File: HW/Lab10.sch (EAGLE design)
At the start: 8 parts, among them Q1 IRLD024

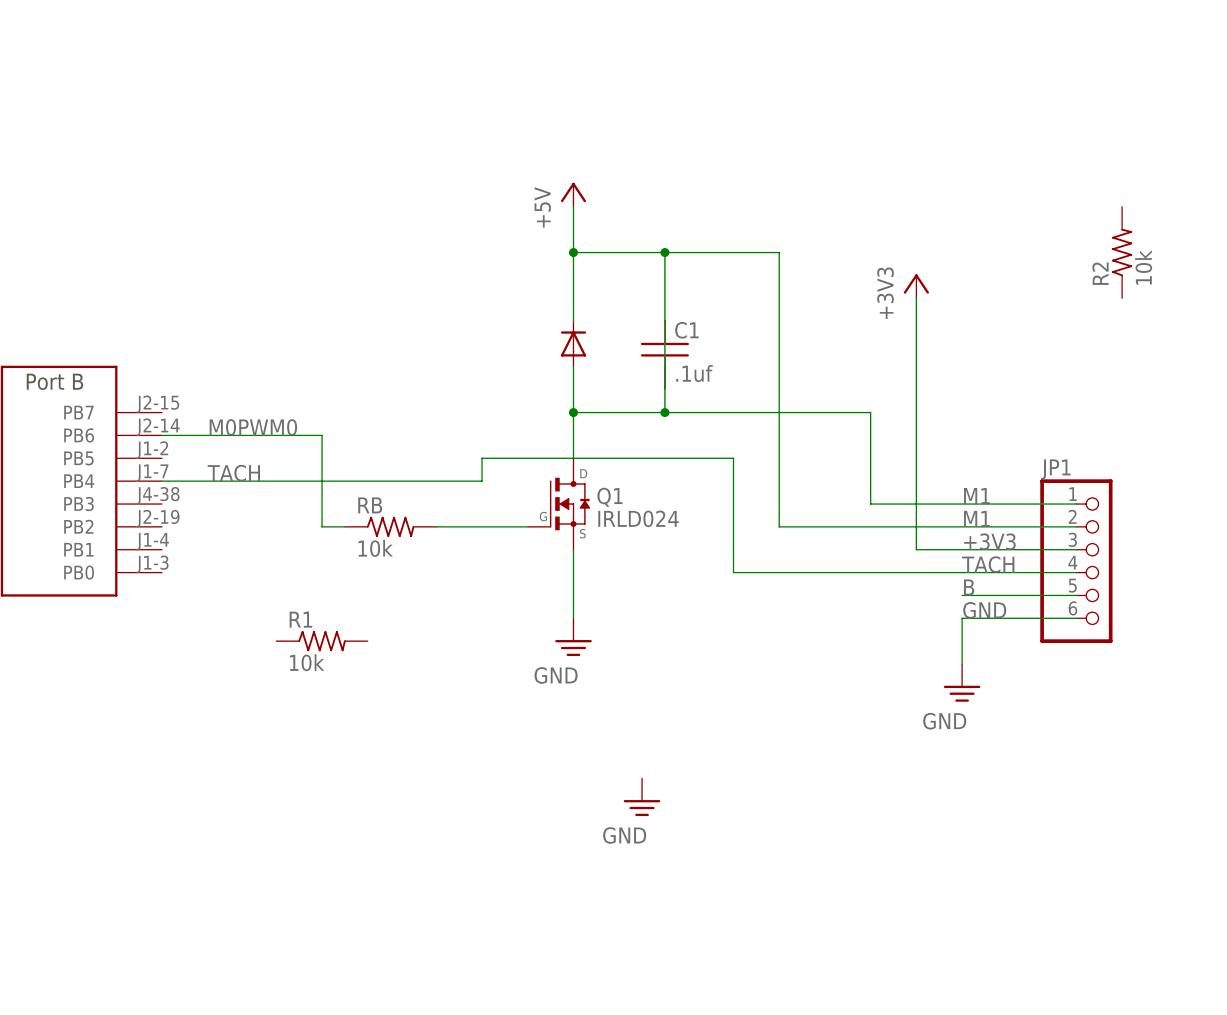
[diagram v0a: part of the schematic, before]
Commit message: Updated HW schematic
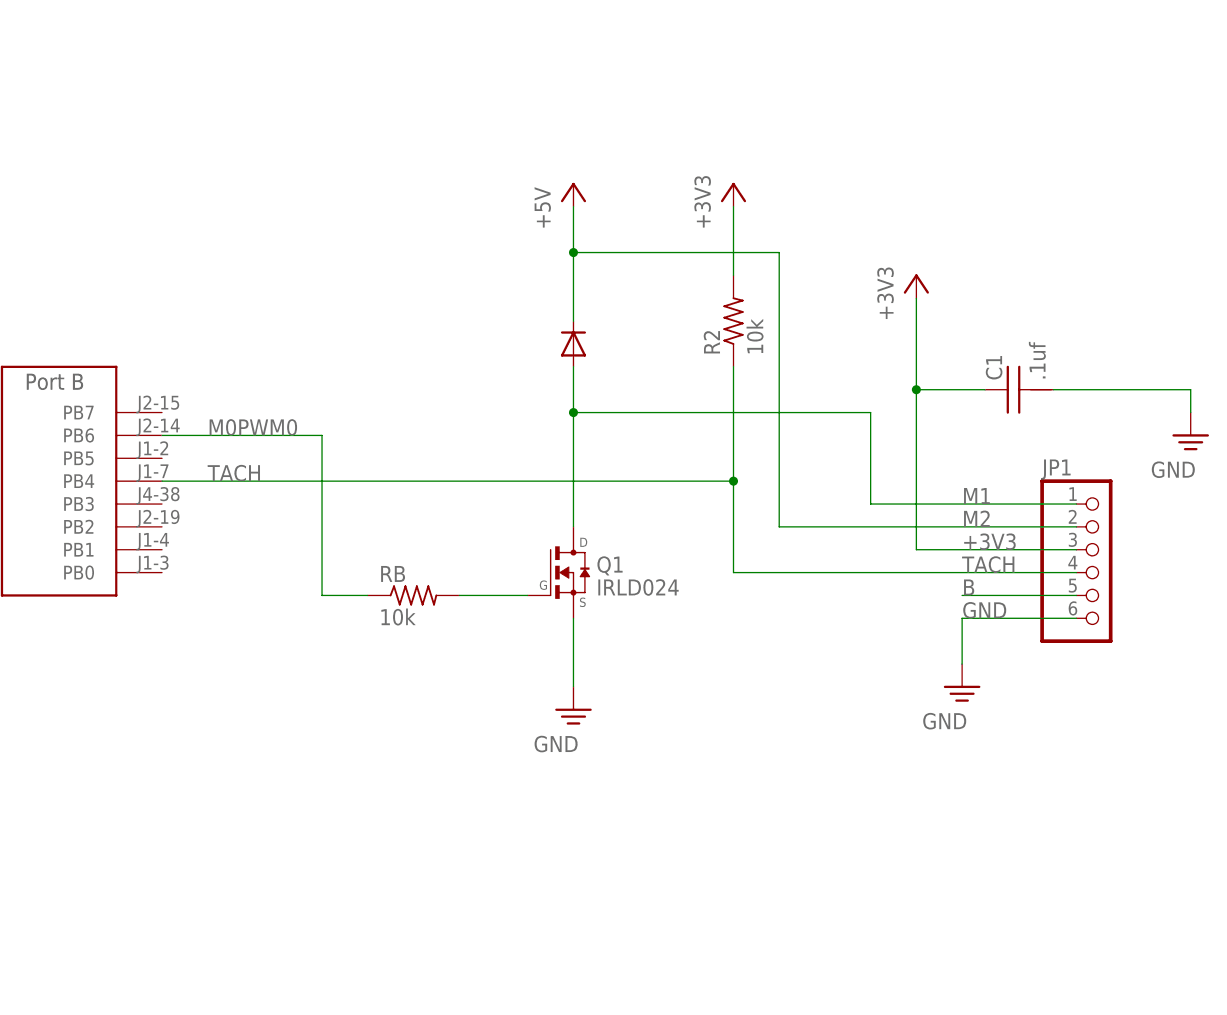
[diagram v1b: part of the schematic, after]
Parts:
- removed R1: 10k, EE445L:RESISTOR0204/5
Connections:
- new net M2: D1.C, JP1.2
- net +3V3: now also C1.1, R2.2
- net GND: now also C1.2
- net M1: no longer C1.1, D1.C, JP1.2
- net TACH: now also R2.1
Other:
- moved on the sheet: C1, Q1, R2, RB
